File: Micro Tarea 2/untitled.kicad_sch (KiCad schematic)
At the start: 43 parts, among them SW1 Reset, SW2 BOOT, U8 ESP32-S3R8, U9 W25Q128JVSIQ, Y1 40MHz

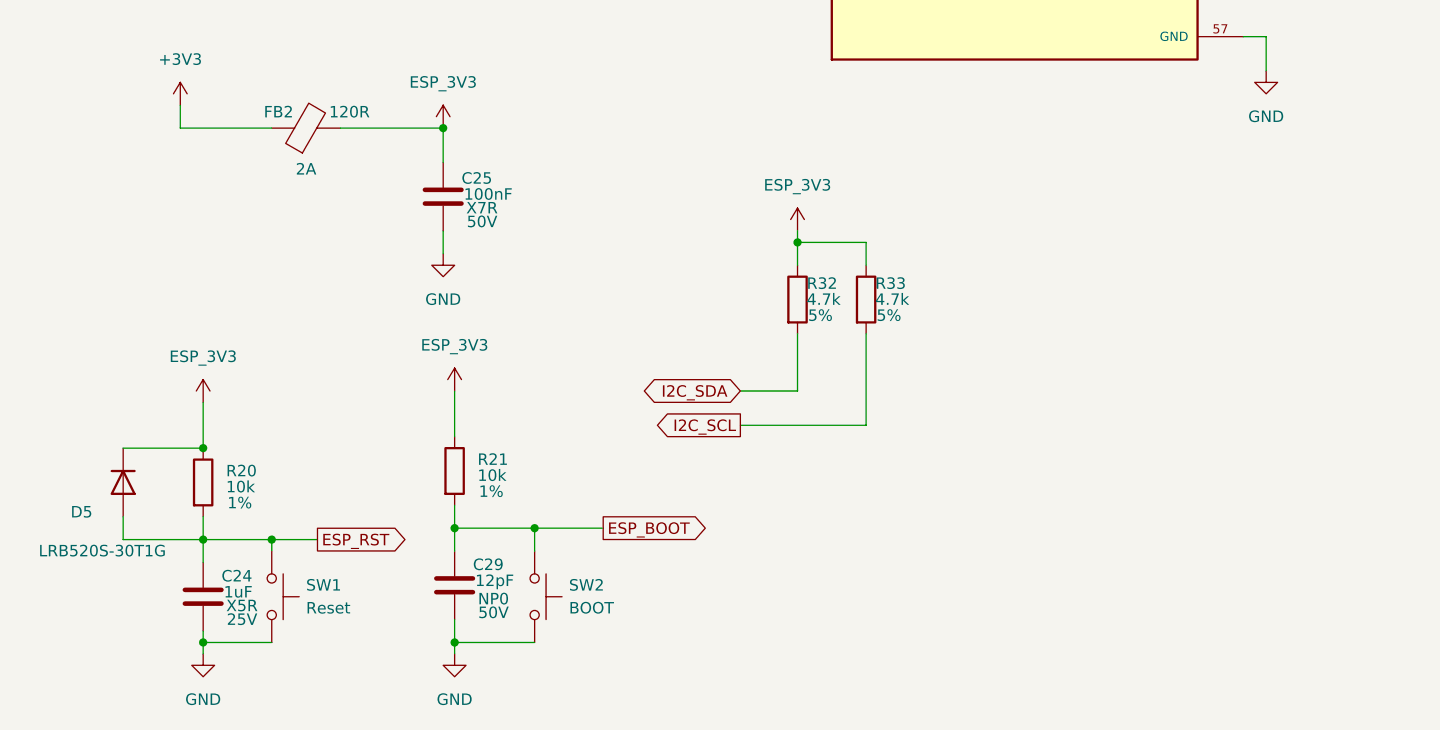
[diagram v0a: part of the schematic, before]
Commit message: actualizando placa
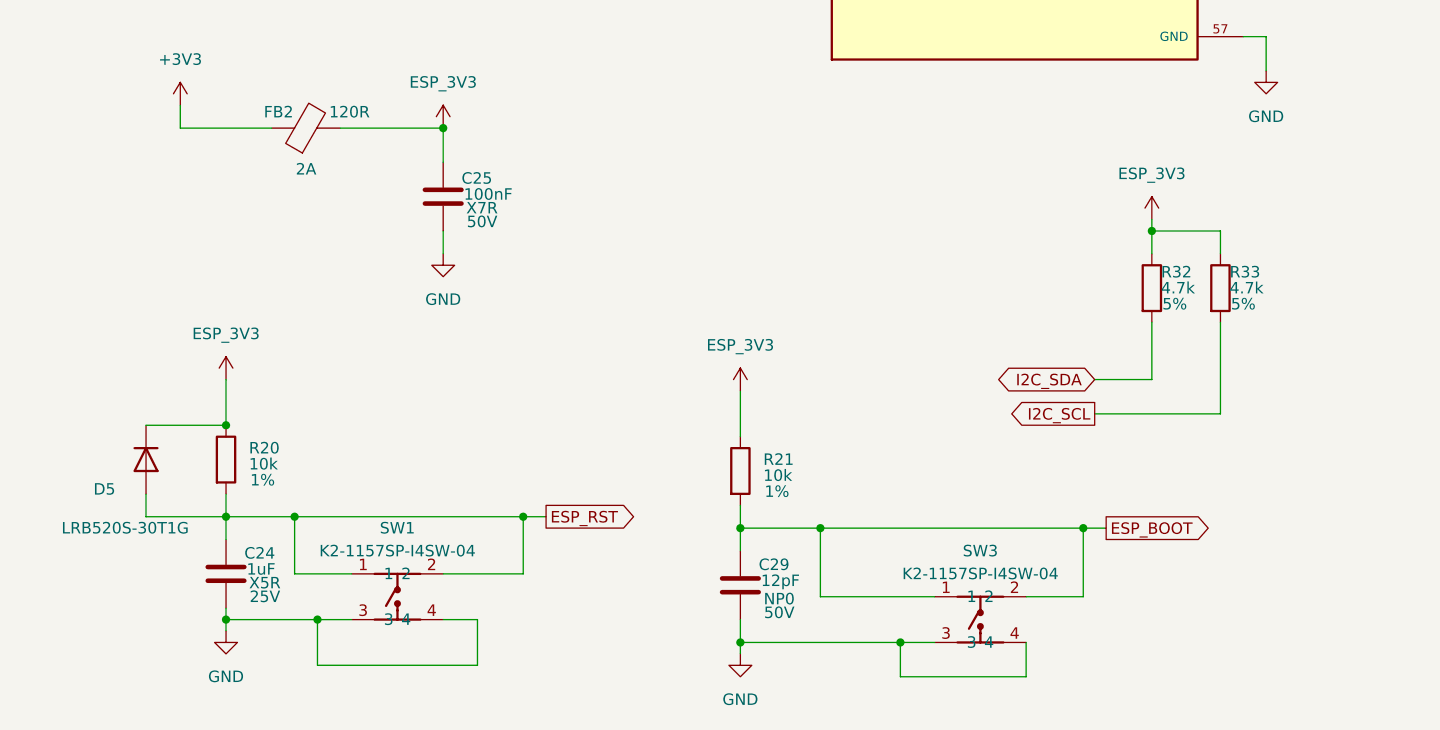
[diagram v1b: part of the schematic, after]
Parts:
- removed SW1: Reset, Onju:SW-SMD_4P-L4.2-W3.2-P2.15-LS4.5, symbol Switch:SW_Push
- removed SW2: BOOT, Onju:SW-SMD_4P-L4.2-W3.2-P2.15-LS4.5, symbol Switch:SW_Push
- added SW1, SW3: K2-1157SP-I4SW-04, JLCImport:K2-1157SP-I4SW-04, symbol JLCImport:K2-1157SP-I4SW-04
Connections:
- net ESP_BOOT: now also SW3.1, SW3.2
- net ESP_RST: now also SW1.1, SW1.2
- net GND: now also SW1.3, SW1.4, SW3.3, SW3.4
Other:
- moved on the sheet: C24, C29, D5, R20, R21, R32, R33
